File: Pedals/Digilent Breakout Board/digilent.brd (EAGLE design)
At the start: 160 x 100 mm, 5 parts

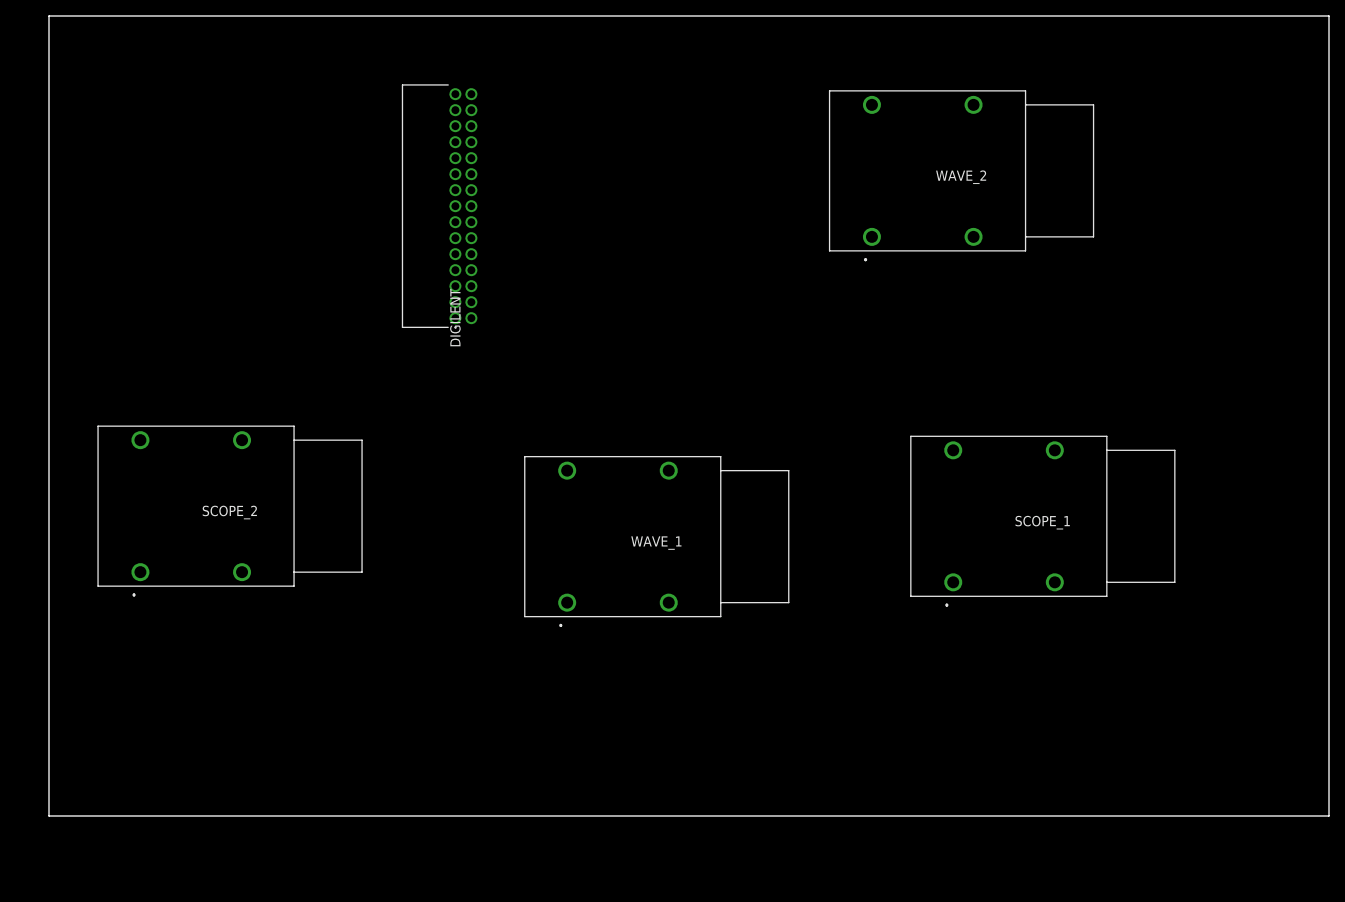
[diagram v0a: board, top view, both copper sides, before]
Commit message: Route board
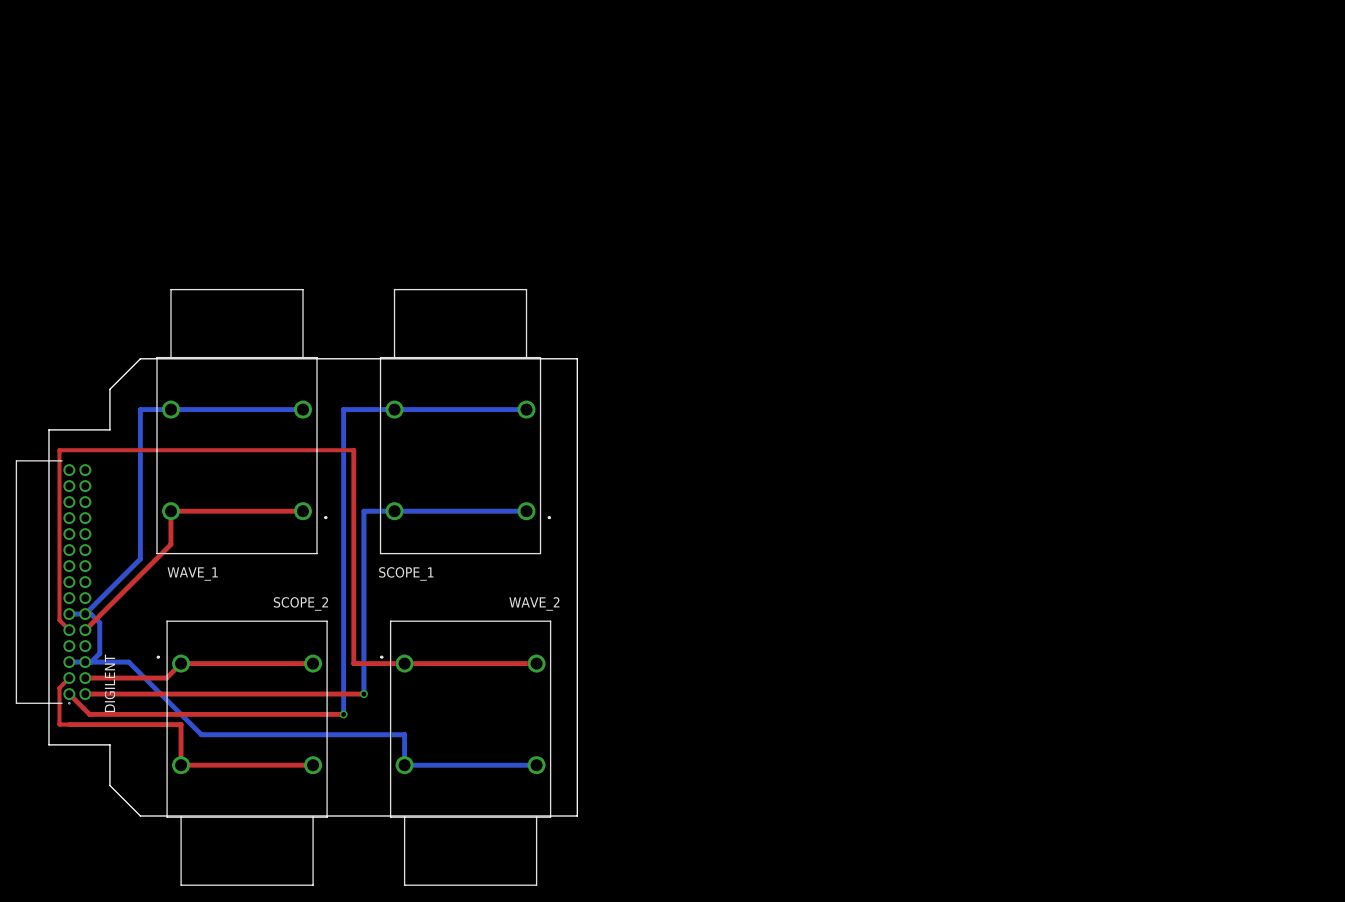
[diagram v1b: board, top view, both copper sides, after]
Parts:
- moved WAVE_2 79.1 mm to (44.5, 19.1), turned to 270 degrees
- moved DIGILENT 67.4 mm to (2.54, 15.2)
- moved SCOPE_1 54.1 mm to (59.7, 38.1), turned to 90 degrees
- moved WAVE_1 34.9 mm to (31.8, 38.1), turned to 90 degrees
- moved SCOPE_2 12.5 mm to (16.5, 19.1), turned to 270 degrees
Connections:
- net N$1 renamed SC1_P
- net N$2 renamed SC2_P
- net N$3 renamed SC1_N
- net N$4 renamed SC2_N
- net N$7 renamed WV_1
- removed net N$5: DIGILENT.9, WAVE_2.3, WAVE_2.4
- new net WV_2: DIGILENT.9, WAVE_2.1, WAVE_2.2
- net AGND: now also WAVE_2.3, WAVE_2.4; no longer WAVE_2.1, WAVE_2.2
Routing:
- net AGND: track 0.00 -> 125.1 mm
- net WV_2: track 0.00 -> 109.3 mm
- net SC1_N: track 0.00 -> 96.3 mm, vias 0 -> 1
- net SC1_P: track 0.00 -> 78.0 mm, vias 0 -> 1
- net SC2_N: track 0.00 -> 43.1 mm
- net WV_1: track 0.00 -> 35.8 mm
- net SC2_P: track 0.00 -> 29.2 mm
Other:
- board size 160 x 100 mm -> 66 x 57.1 mm
